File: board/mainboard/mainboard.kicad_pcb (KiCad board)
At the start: 2 copper layers, 148.1 x 58.4 mm, 97 parts, among them J1 BACKL, P1 I2C, P10 BUMPERS, P12 POWER, P2 Motor1, P3 Motor2, P4 SPI, P5 DAC, P6 LINE SENSORS, P7 ANALOG, P8 OPTIONAL PERIPHERALS, P9 GPIO, SW1 SW_PUSH, SW2 SW_PUSH, SW3 SW_PUSH, SW4 SW_PUSH, U1 74LS138, U2 74ALVC125, U3 74ALVC126, U4 74ALVC126, U5 74ALVC126, U6 PCA9515B, X1 32.768KHz, X2 12.288MHz

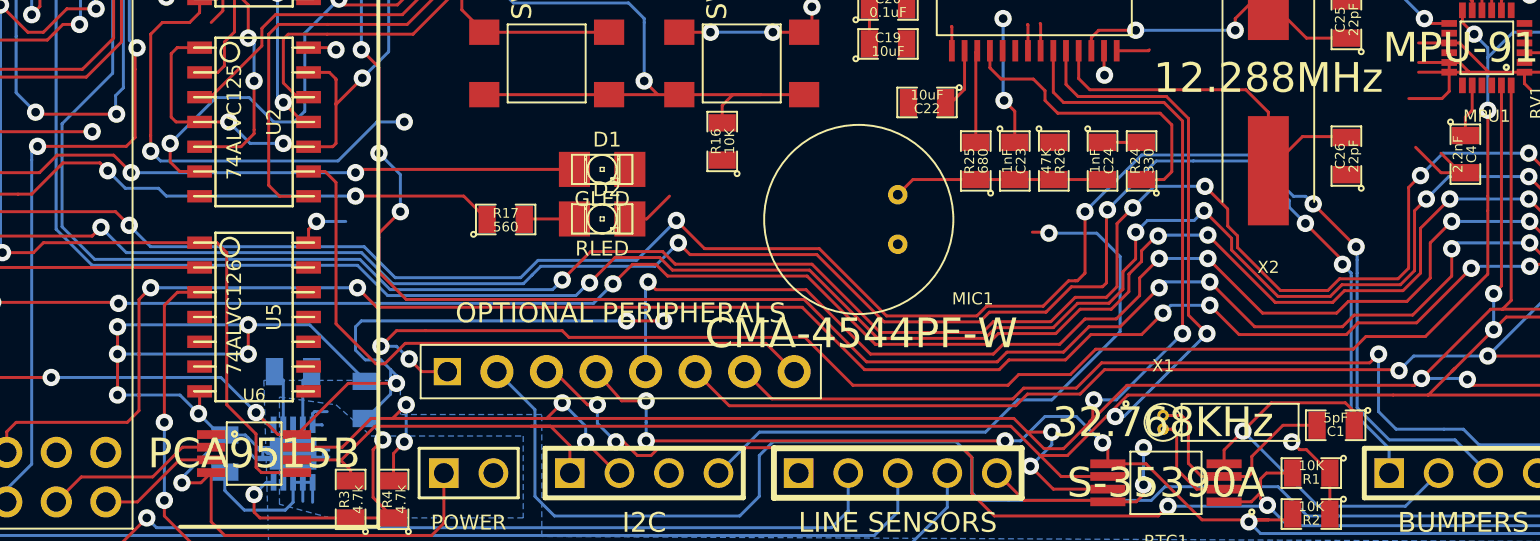
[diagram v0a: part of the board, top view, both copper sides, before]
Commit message: Cleaning up busses
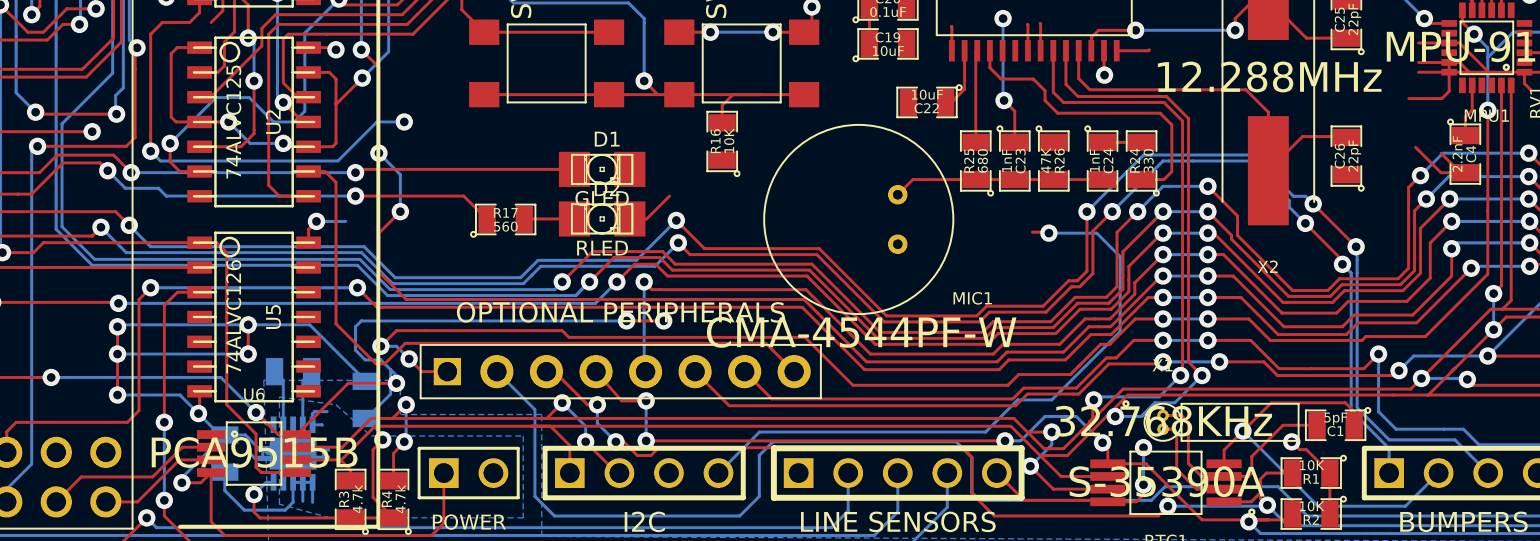
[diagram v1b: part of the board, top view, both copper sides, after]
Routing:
- net I2C_CL: track 199.6 -> 201.5 mm
- net I2C_DA: track 209.6 -> 211.0 mm
- net MOTOR2F: track 117.1 -> 118.3 mm, vias 3 -> 5
- net MOTOR1F: track 114.9 -> 116.0 mm, vias 4 -> 6
- net MPUINT: track 119.7 -> 120.6 mm, vias 5 -> 7
- net BUMP1: track 138.5 -> 137.6 mm
- net SPI_SEL2: track 181.6 -> 181.1 mm
- net SPI_SEL1: track 176.5 -> 177.0 mm
